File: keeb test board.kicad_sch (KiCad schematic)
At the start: 15 parts, among them SW12 SW_Push, SW14 SW_Push, SW15 SW_Push, SW3 SW_Push, SW6 SW_Push, SW9 SW_Push, U1 BluePill_V1.1

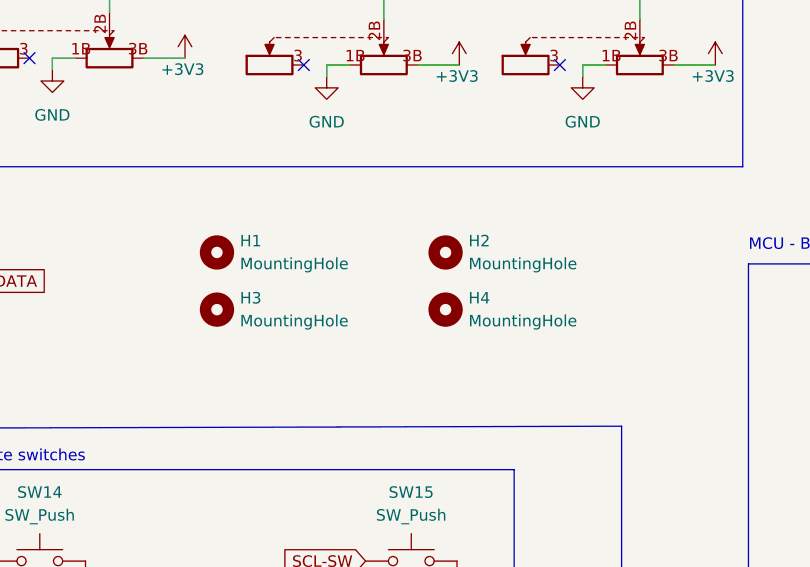
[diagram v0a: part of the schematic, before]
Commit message: Routing improvements
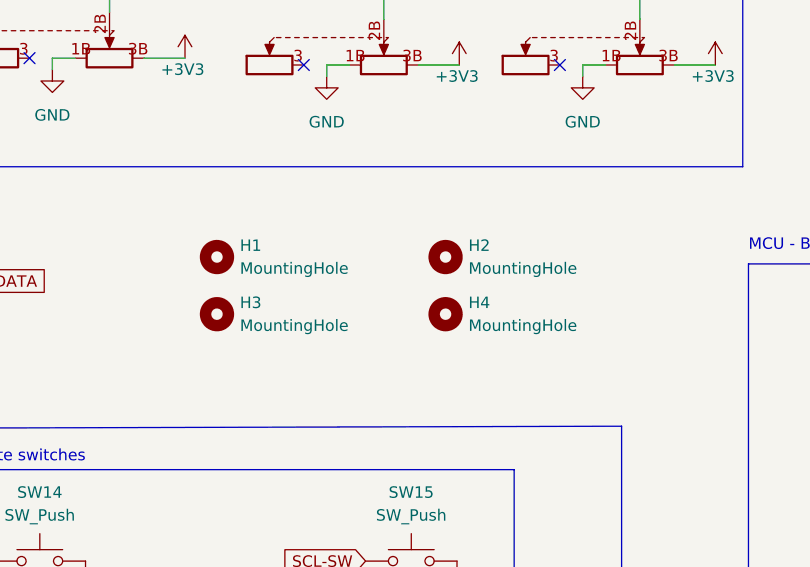
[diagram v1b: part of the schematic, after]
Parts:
- H1, H2, H3, H4: footprint MountingHole:MountingHole_2.2mm_M2_DIN965 -> Keeby-Cat Footprints:MountingHole_2.2mm_M2_DIN965
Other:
- moved on the sheet: H1, H2, H3, H4
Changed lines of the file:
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@@
     (pin "1")
   )
-  (symbol (lib_id "Mechanical:MountingHole") (at 135.89 64.77 0) (unit 1)
-    (in_bom yes) (on_board yes) (fields_autoplaced)
-    (property "Reference" "H2" (id 0) (at 138.43 63.4999 0)
-      (effects (font (size 1.27 1.27)) (justify left))
-    )
-    (property "Value" "MountingHole" (id 1) (at 138.43 66.0399 0)
-      (effects (font (size 1.27 1.27)) (justify left))
-    )
-    (property "Footprint" "MountingHole:MountingHole_2.2mm_M2_DIN965" (id 2) (at 135.89 64.77 0)
-      (effects (font (size 1.27 1.27)) hide)
-    )
-    (property "Datasheet" "~" (id 3) (at 135.89 64.77 0)
+  (symbol (lib_id "Mechanical:MountingHole") (at 135.89 65.278 0) (unit 1)
+    (in_bom yes) (on_board yes) (fields_autoplaced)
+    (property "Reference" "H2" (id 0) (at 138.43 64.0079 0)
+      (effects (font (size 1.27 1.27)) (justify left))
+    )
+    (property "Value" "MountingHole" (id 1) (at 138.43 66.5479 0)
+      (effects (font (size 1.27 1.27)) (justify left))
+    )
+    (property "Footprint" "Keeby-Cat Footprints:MountingHole_2.2mm_M2_DIN965" (id 2) (at 135.89 65.278 0)
+      (effects (font (size 1.27 1.27)) hide)
+    )
+    (property "Datasheet" "~" (id 3) (at 135.89 65.278 0)
       (effects (font (size 1.27 1.27)) hide)
     )
@@
     (pin "4")
   )
-  (symbol (lib_id "Mechanical:MountingHole") (at 135.89 71.12 0) (unit 1)
-    (in_bom yes) (on_board yes) (fields_autoplaced)
-    (property "Reference" "H4" (id 0) (at 138.43 69.8499 0)
-      (effects (font (size 1.27 1.27)) (justify left))
-    )
-    (property "Value" "MountingHole" (id 1) (at 138.43 72.3899 0)
-      (effects (font (size 1.27 1.27)) (justify left))
-    )
-    (property "Footprint" "MountingHole:MountingHole_2.2mm_M2_DIN965" (id 2) (at 135.89 71.12 0)
-      (effects (font (size 1.27 1.27)) hide)
-    )
-    (property "Datasheet" "~" (id 3) (at 135.89 71.12 0)
+  (symbol (lib_id "Mechanical:MountingHole") (at 135.89 71.628 0) (unit 1)
+    (in_bom yes) (on_board yes) (fields_autoplaced)
+    (property "Reference" "H4" (id 0) (at 138.43 70.3579 0)
+      (effects (font (size 1.27 1.27)) (justify left))
+    )
+    (property "Value" "MountingHole" (id 1) (at 138.43 72.8979 0)
+      (effects (font (size 1.27 1.27)) (justify left))
+    )
+    (property "Footprint" "Keeby-Cat Footprints:MountingHole_2.2mm_M2_DIN965" (id 2) (at 135.89 71.628 0)
+      (effects (font (size 1.27 1.27)) hide)
+    )
+    (property "Datasheet" "~" (id 3) (at 135.89 71.628 0)
       (effects (font (size 1.27 1.27)) hide)
     )
@@
     (pin "2")
   )
-  (symbol (lib_id "Mechanical:MountingHole") (at 110.49 64.77 0) (unit 1)
-    (in_bom yes) (on_board yes) (fields_autoplaced)
-    (property "Reference" "H1" (id 0) (at 113.03 63.4999 0)
-      (effects (font (size 1.27 1.27)) (justify left))
-    )
-    (property "Value" "MountingHole" (id 1) (at 113.03 66.0399 0)
-      (effects (font (size 1.27 1.27)) (justify left))
-    )
-    (property "Footprint" "MountingHole:MountingHole_2.2mm_M2_DIN965" (id 2) (at 110.49 64.77 0)
-      (effects (font (size 1.27 1.27)) hide)
-    )
-    (property "Datasheet" "~" (id 3) (at 110.49 64.77 0)
+  (symbol (lib_id "Mechanical:MountingHole") (at 110.49 65.278 0) (unit 1)
+    (in_bom yes) (on_board yes) (fields_autoplaced)
+    (property "Reference" "H1" (id 0) (at 113.03 64.0079 0)
+      (effects (font (size 1.27 1.27)) (justify left))
+    )
+    (property "Value" "MountingHole" (id 1) (at 113.03 66.5479 0)
+      (effects (font (size 1.27 1.27)) (justify left))
+    )
+    (property "Footprint" "Keeby-Cat Footprints:MountingHole_2.2mm_M2_DIN965" (id 2) (at 110.49 65.278 0)
+      (effects (font (size 1.27 1.27)) hide)
+    )
+    (property "Datasheet" "~" (id 3) (at 110.49 65.278 0)
       (effects (font (size 1.27 1.27)) hide)
     )
@@
     (pin "1")
   )
-  (symbol (lib_id "Mechanical:MountingHole") (at 110.49 71.12 0) (unit 1)
-    (in_bom yes) (on_board yes) (fields_autoplaced)
-    (property "Reference" "H3" (id 0) (at 113.03 69.8499 0)
-      (effects (font (size 1.27 1.27)) (justify left))
-    )
-    (property "Value" "MountingHole" (id 1) (at 113.03 72.3899 0)
-      (effects (font (size 1.27 1.27)) (justify left))
-    )
-    (property "Footprint" "MountingHole:MountingHole_2.2mm_M2_DIN965" (id 2) (at 110.49 71.12 0)
-      (effects (font (size 1.27 1.27)) hide)
-    )
-    (property "Datasheet" "~" (id 3) (at 110.49 71.12 0)
+  (symbol (lib_id "Mechanical:MountingHole") (at 110.49 71.628 0) (unit 1)
+    (in_bom yes) (on_board yes) (fields_autoplaced)
+    (property "Reference" "H3" (id 0) (at 113.03 70.3579 0)
+      (effects (font (size 1.27 1.27)) (justify left))
+    )
+    (property "Value" "MountingHole" (id 1) (at 113.03 72.8979 0)
+      (effects (font (size 1.27 1.27)) (justify left))
+    )
+    (property "Footprint" "Keeby-Cat Footprints:MountingHole_2.2mm_M2_DIN965" (id 2) (at 110.49 71.628 0)
+      (effects (font (size 1.27 1.27)) hide)
+    )
+    (property "Datasheet" "~" (id 3) (at 110.49 71.628 0)
       (effects (font (size 1.27 1.27)) hide)
     )
@@
     )
     (path "/d7dc8332-4e7d-4d1c-9e13-94700025e229"
-      (reference "H1") (unit 1) (value "MountingHole") (footprint "MountingHole:MountingHole_2.2mm_M2_DIN965")
+      (reference "H1") (unit 1) (value "MountingHole") (footprint "Keeby-Cat Footprints:MountingHole_2.2mm_M2_DIN965")
     )
     (path "/5a7e5e4b-0f2c-4c71-9d32-45cf0732b0c3"
-      (reference "H2") (unit 1) (value "MountingHole") (footprint "MountingHole:MountingHole_2.2mm_M2_DIN965")
+      (reference "H2") (unit 1) (value "MountingHole") (footprint "Keeby-Cat Footprints:MountingHole_2.2mm_M2_DIN965")
     )
     (path "/f81e2caa-f7a2-40dd-8668-c447b8223c0a"
-      (reference "H3") (unit 1) (value "MountingHole") (footprint "MountingHole:MountingHole_2.2mm_M2_DIN965")
+      (reference "H3") (unit 1) (value "MountingHole") (footprint "Keeby-Cat Footprints:MountingHole_2.2mm_M2_DIN965")
     )
     (path "/8ea18563-8d92-48ab-81f4-e90c6181f6de"
-      (reference "H4") (unit 1) (value "MountingHole") (footprint "MountingHole:MountingHole_2.2mm_M2_DIN965")
+      (reference "H4") (unit 1) (value "MountingHole") (footprint "Keeby-Cat Footprints:MountingHole_2.2mm_M2_DIN965")
     )
     (path "/6ce8230c-595b-49b4-b7e1-27c56bb79809/368da0b2-4a09-4c1c-a7bd-9829d431f181"
